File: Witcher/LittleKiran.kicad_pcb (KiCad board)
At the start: 2 copper layers, 36.1 x 36.1 mm, 18 parts, among them J1 XT60PW-M, J2 XT60PW-M, J3 XT60PW-M, Q1 PXP012-30QLJ, Q2 PXP012-30QLJ, Q3 PXP012-30QLJ, Q4 FDN340P, U1 LTC4412xS6, U2 LTC4412xS6

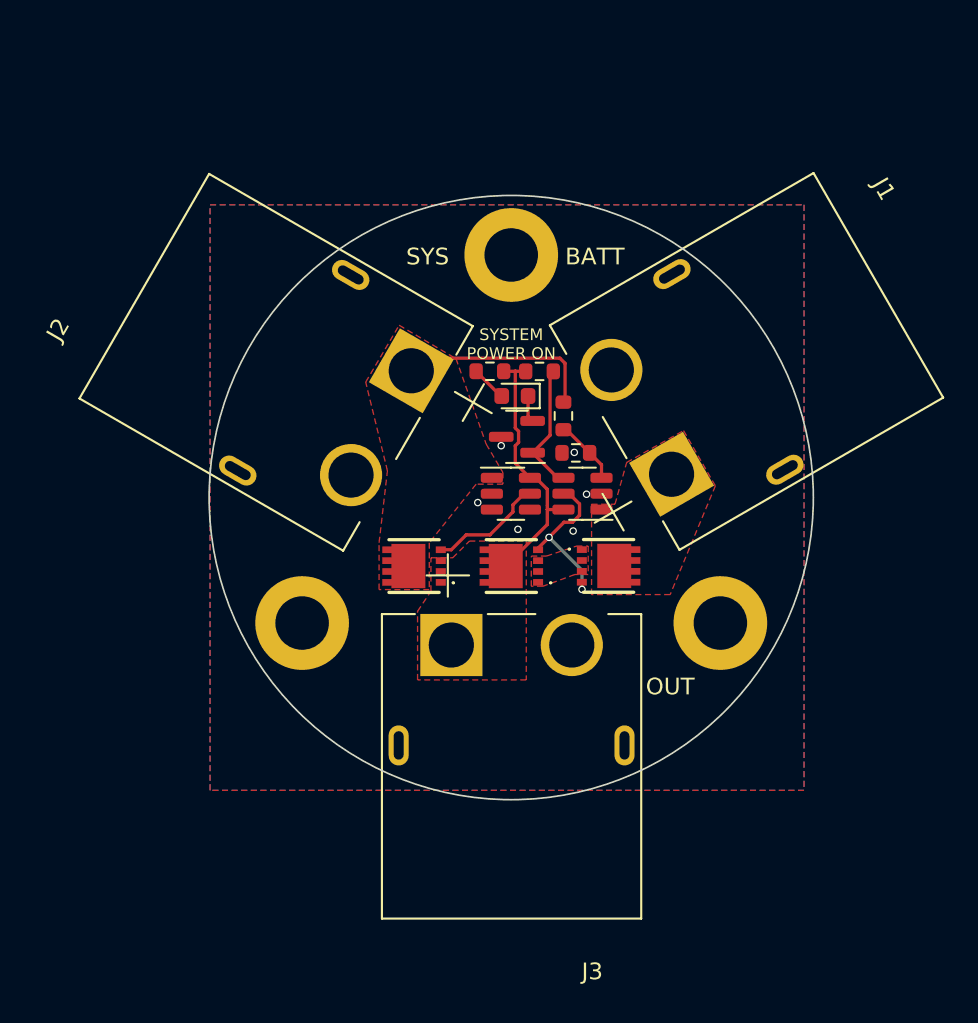
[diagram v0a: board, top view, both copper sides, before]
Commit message: kiran fixes
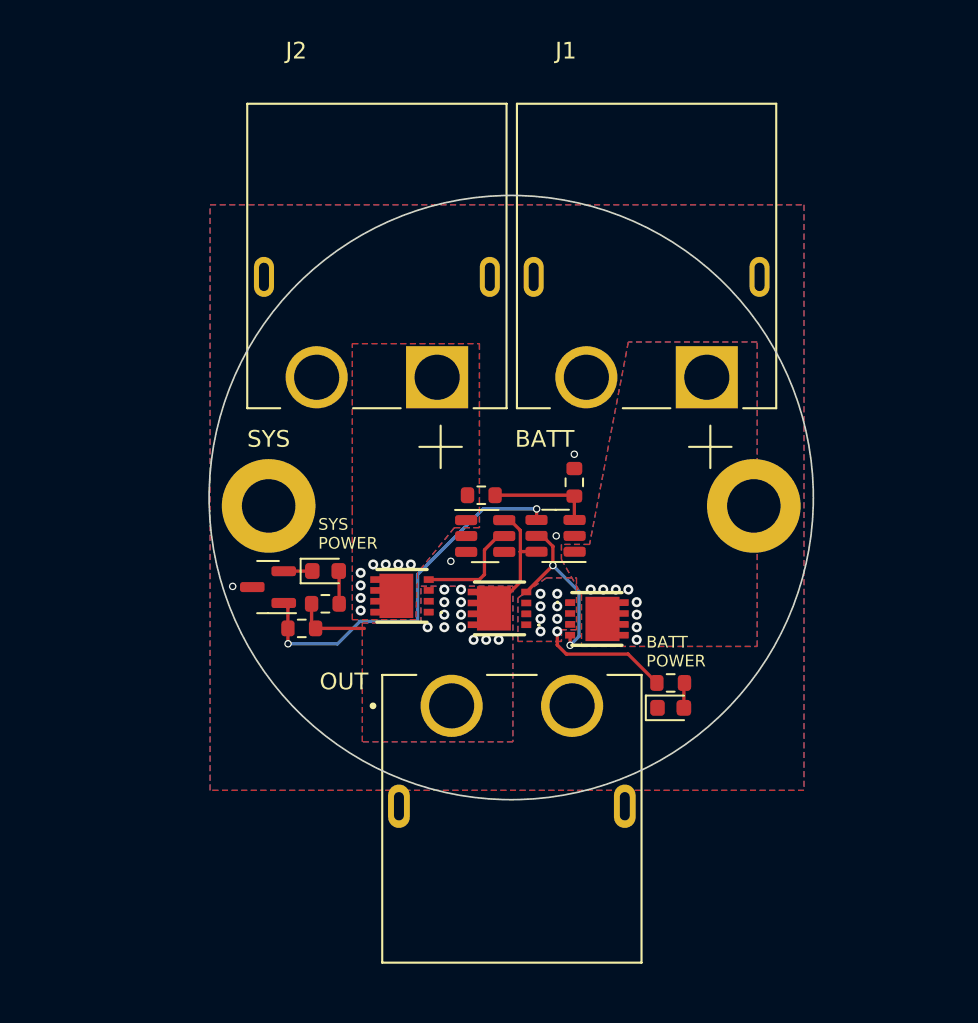
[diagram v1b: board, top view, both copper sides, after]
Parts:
- removed H2: MountingHole_Pad, MountingHole:MountingHole_3.2mm_M3_DIN965_Pad
- added D2: BATT_LED, LED_SMD:LED_0603_1608Metric, F.Cu at (139.0, 94.1)
- added R5: 3k, Resistor_SMD:R_0603_1608Metric, F.Cu at (139.0, 92.6)
- J3: value XT60PW-M -> XT60PW-F; footprint iclr:AMASS_XT60PW-M -> iclr:AMASS_XT60PW-F
- moved R3 20.9 mm to (117.0, 89.3), turned to 180 degrees
- moved Q4 17.4 mm to (115.0, 86.8)
- moved R4 17.0 mm to (118.4, 87.8), turned to 0 degrees
- moved D1 15.4 mm to (118.4, 85.9), turned to 0 degrees
- moved J2 7.57 mm to (121.5, 68.3), turned to 0 degrees
- moved J1 7.49 mm to (137.6, 68.3), turned to 0 degrees
- moved H1 7.28 mm to (144.0, 82.0)
- moved H3 7.28 mm to (115.0, 82.0)
- moved R1 6.82 mm to (127.7, 81.4), turned to 180 degrees
- moved Q2 3.25 mm to (134.6, 88.8)
- moved U1 2.99 mm to (132.2, 83.8)
- moved U2 2.96 mm to (127.9, 83.8)
- moved Q3 2.63 mm to (128.8, 88.1)
- moved J3 2.36 mm to (129.5, 94.0), turned to 0 degrees
- moved Q1 1.92 mm to (123.0, 87.4)
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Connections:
- J3 pad S1: (no net) -> unconnected-(J3-SHIELD-PadS1)
- J3 pad S2: (no net) -> unconnected-(J3-SHIELD-PadS1)
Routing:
- net /STAT: track 7.84 -> 23.0 mm, vias 0 -> 2
- net Net-(J2-+): track 12.0 -> 0.00 mm, vias 0 -> 8
- net Net-(Q2-S_1): track 0.00 -> 7.71 mm, vias 0 -> 8
- net /SENSE: track 16.1 -> 12.0 mm, vias 0 -> 12
- net Net-(U1-CTL): track 3.92 -> 6.19 mm
- net Net-(D2-A): track 0.00 -> 1.51 mm
- net /GATE1: track 9.64 -> 10.9 mm
- net Net-(Q1-G): track 6.96 -> 6.45 mm
- net Net-(J1-+): vias 0 -> 8
- net GND: vias 6 -> 4
- added copper zone on B.Cu, net /SENSE
- added copper zone on B.Cu, net Net-(J1-+)
- added copper zone on B.Cu, net Net-(J2-+)
- added copper zone on B.Cu, net Net-(Q2-S_1)
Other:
- board text added: "BATT POWER"
- board text added: "SYS POWER"
- board text removed: "SYSTEM POWER ON"

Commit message: update
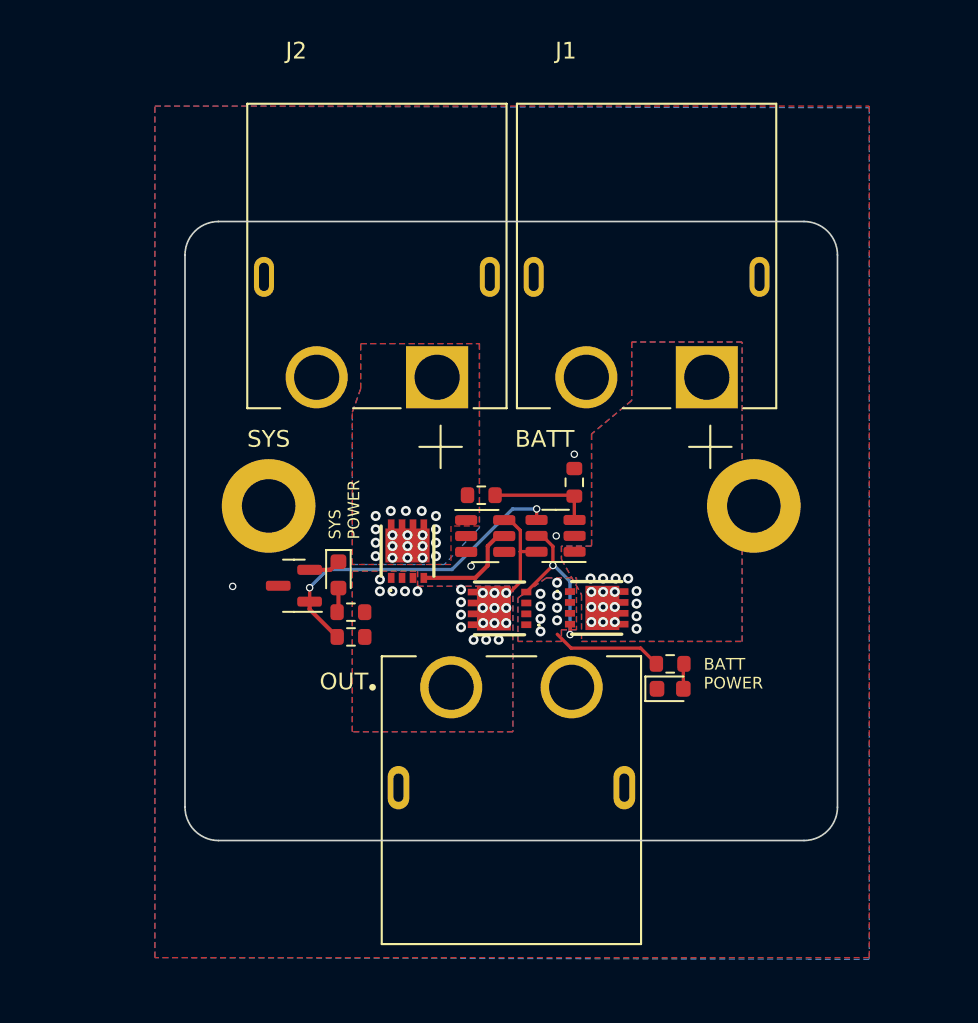
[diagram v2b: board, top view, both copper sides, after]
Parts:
- moved R3 2.98 mm to (119.9, 89.8)
- moved Q1 2.70 mm to (123.3, 84.7), turned to 0 degrees
- moved R4 1.60 mm to (119.9, 88.3), turned to 180 degrees
- moved Q4 1.55 mm to (116.5, 86.8)
- moved R5 1.14 mm to (139.0, 91.4)
- moved D2 1.14 mm to (139.0, 92.9)
- moved J3 1.11 mm to (129.5, 92.8)
- moved D1 0.81 mm to (119.2, 86.1), turned to -90 degrees
- moved Q2 0.66 mm to (134.6, 88.1)
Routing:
- net /SENSE: track 12.0 -> 7.51 mm, vias 12 -> 21
- net /STAT: track 23.0 -> 19.8 mm
- net Net-(Q2-S_1): track 7.71 -> 6.66 mm
- net /GATE1: track 10.9 -> 9.85 mm
- net Net-(J2-+): vias 8 -> 20
- net Net-(J1-+): vias 8 -> 17
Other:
- board size 36.1 x 36.1 mm -> 39 x 37 mm
